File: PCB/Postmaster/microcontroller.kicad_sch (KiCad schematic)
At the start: 25 parts, among them J1 Conn_01x02, J2 Conn_02x08_Odd_Even, J3 Conn_01x04, J4 Conn_01x04, J5 Conn_01x03, J6 Conn_02x10_Odd_Even, U2 STM32F407VETx, U3 S25FL064LABMFI013, Y1 TFOM50M4RWKCKT2T, Y2 CSTNE8M00G550000R0

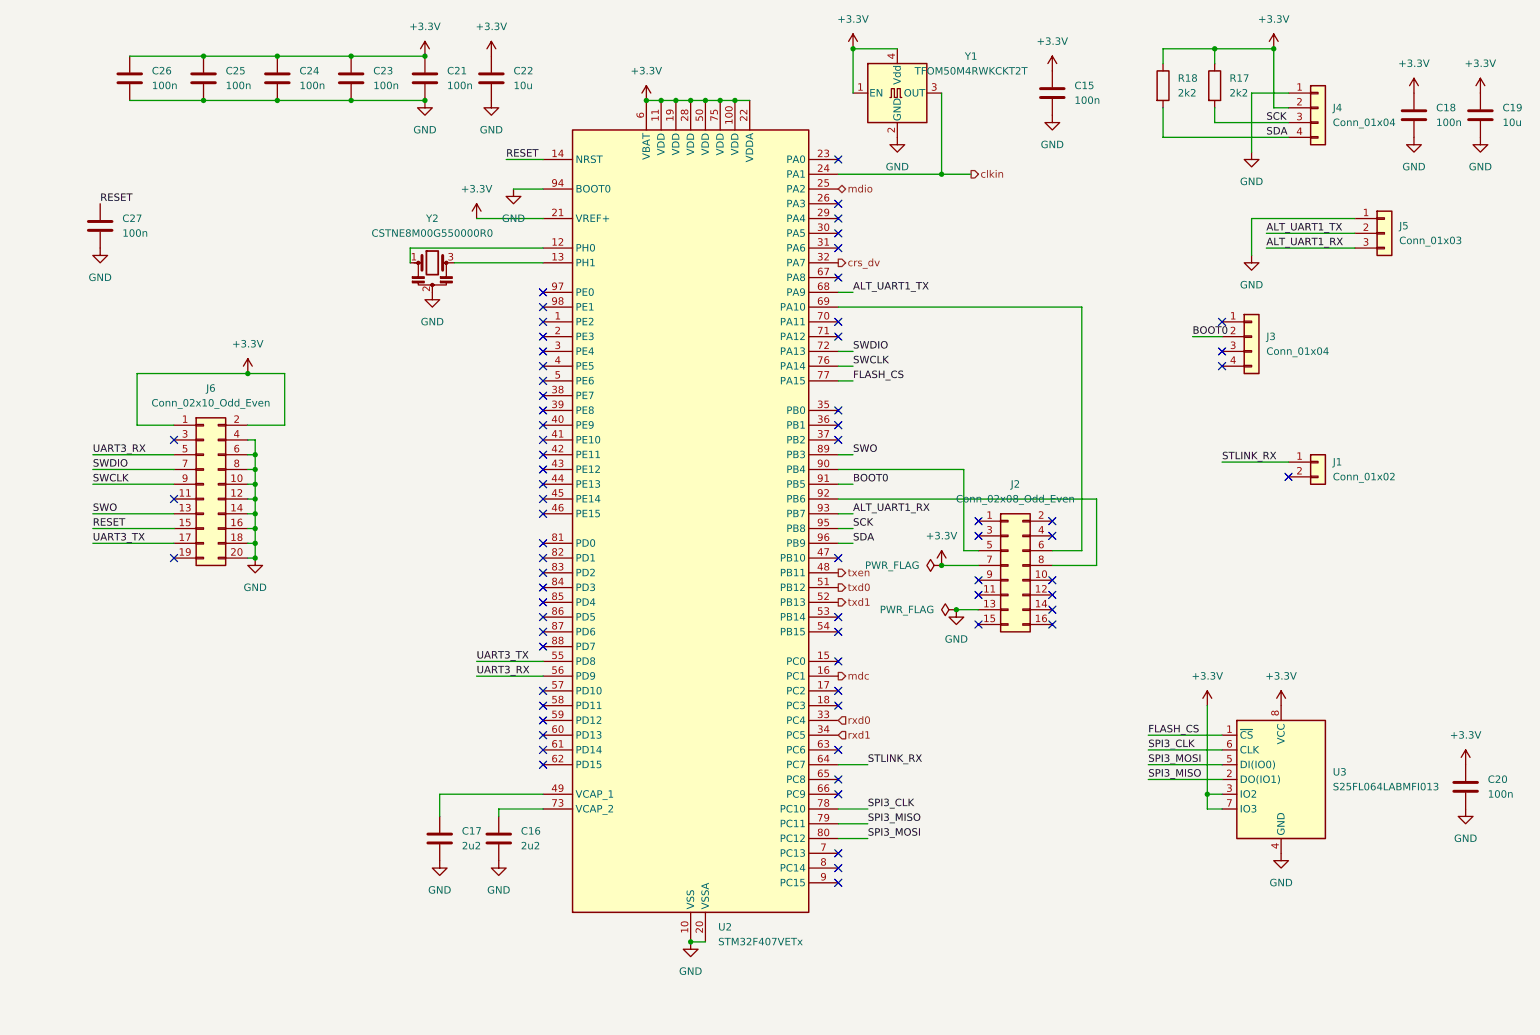
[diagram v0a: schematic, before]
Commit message: Update schematics
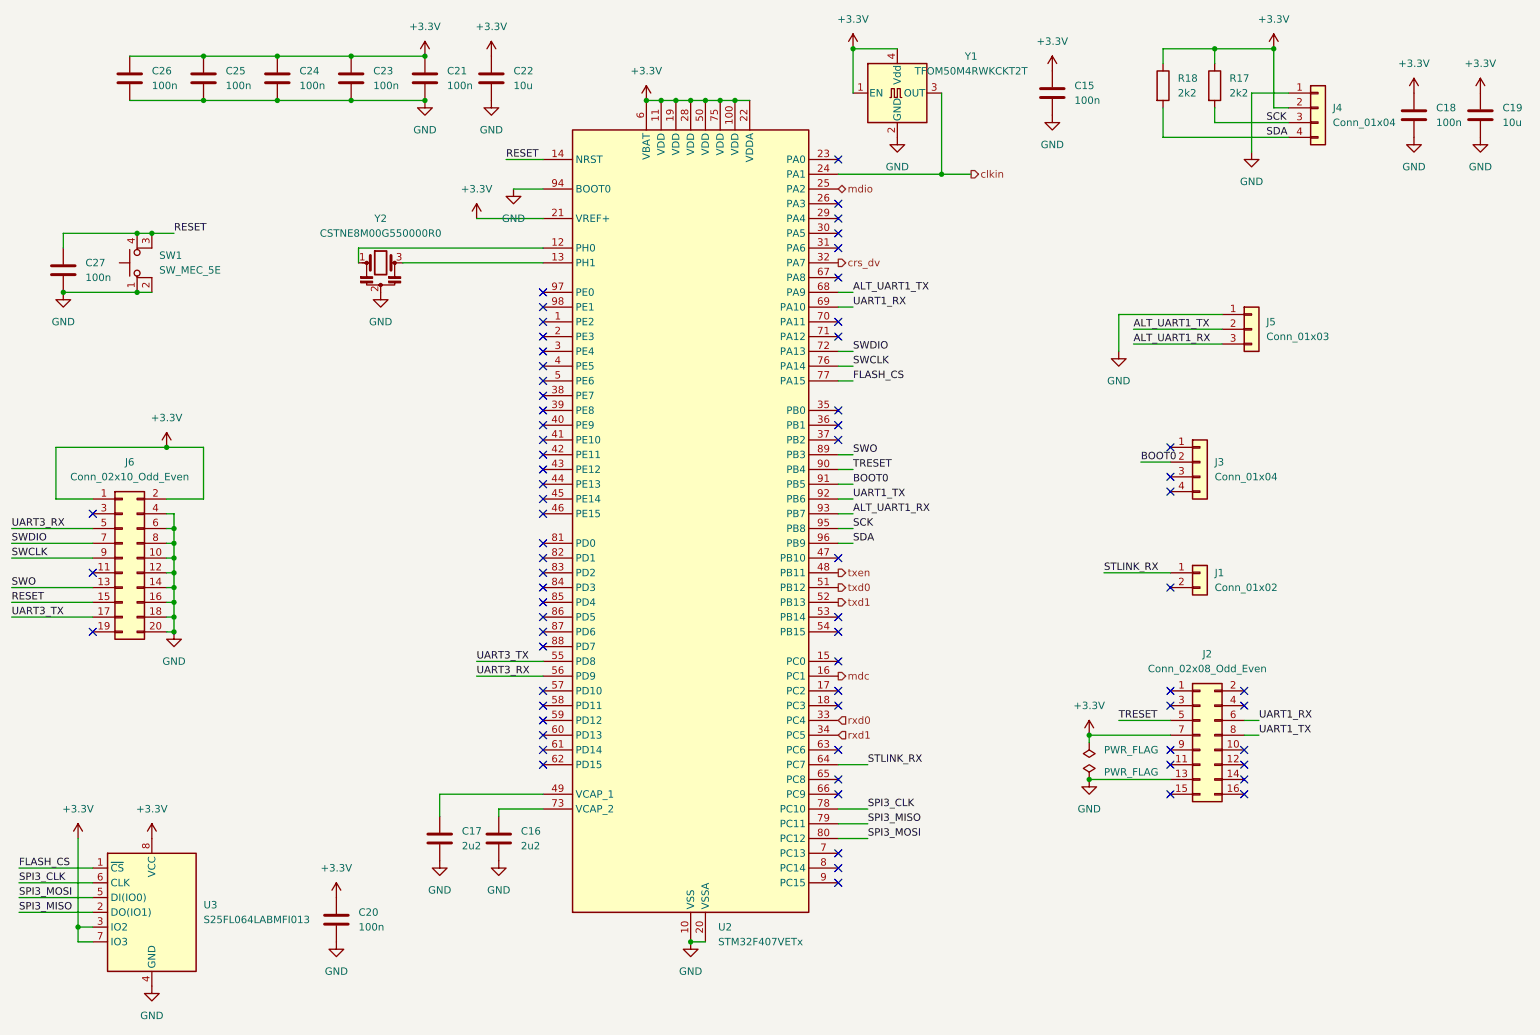
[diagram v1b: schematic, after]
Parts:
- added SW1: SW_MEC_5E, Button_Switch_SMD:SW_SPST_TL3305B, symbol Switch:SW_MEC_5E
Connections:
- net GND: now also SW1.1, SW1.2
- net RESET: now also SW1.3 (K), SW1.4 (A)
- net TRESET: now reaches J2.5 (Pin_5), U2.90 (PB4)
- net UART1_RX: now reaches J2.6 (Pin_6), U2.69 (PA10)
- net UART1_TX: now reaches J2.8 (Pin_8), U2.92 (PB6)
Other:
- moved on the sheet: C20, C27, J1, J2, J3, J5, J6, U3, Y2
